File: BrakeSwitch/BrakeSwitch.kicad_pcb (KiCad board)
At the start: 2 copper layers, 16 parts, among them Q1 NMOS, U1 XL1509-5.0, U2 LMV321, U3 LMV321

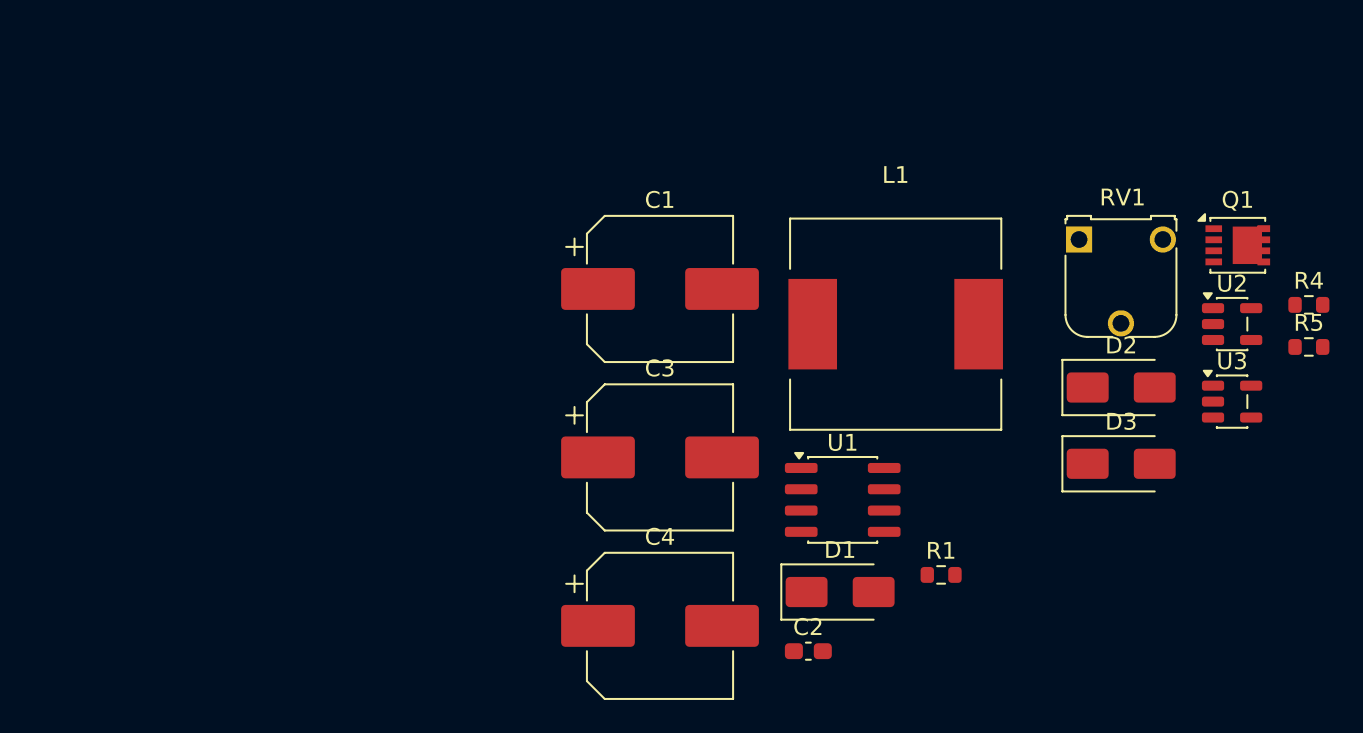
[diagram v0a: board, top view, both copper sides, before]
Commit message: Basic layout done
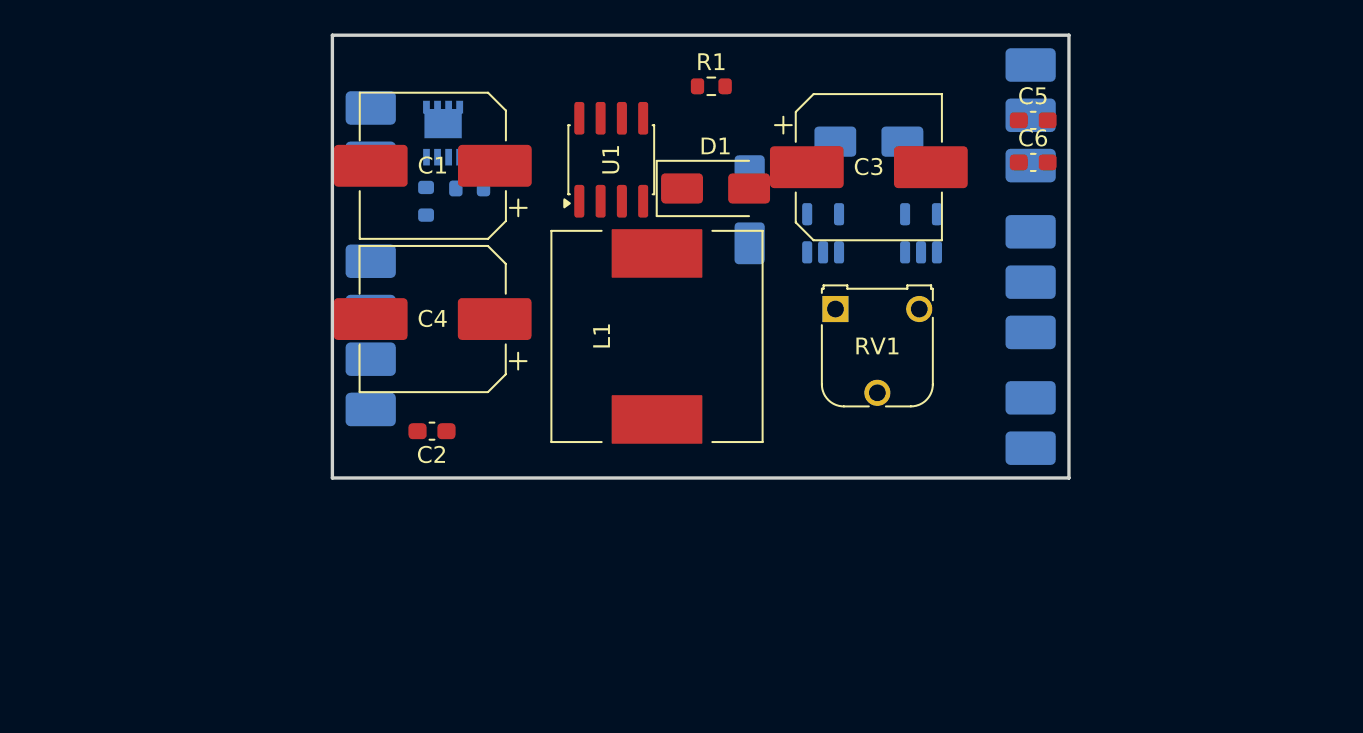
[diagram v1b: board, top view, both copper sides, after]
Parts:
- added C5: 1u, Capacitor_SMD:C_0603_1608Metric_Pad1.08x0.95mm_HandSolder, F.Cu at (114.2, 38.9)
- added C6: 1u, Capacitor_SMD:C_0603_1608Metric_Pad1.08x0.95mm_HandSolder, F.Cu at (114.2, 41.4)
- added J1: 12V_in, AA-Custom:SolderPad_01x02, B.Cu at (74.7, 48.8)
- added J2: LightPlug, AA-Custom:SolderPad_01x02, B.Cu at (74.7, 39.6)
- added J3: 5V_out, AA-Custom:SolderPad_01x02, B.Cu at (114.0, 56.9)
- added J4: Front_Pads, AA-Custom:SolderPad_01x03, B.Cu at (114.0, 48.5)
- added J5: Back_Pads, AA-Custom:SolderPad_01x03, B.Cu at (114.0, 38.6)
- added J6: 12V_in, AA-Custom:SolderPad_01x02, B.Cu at (74.7, 54.6)
- D2, D3, Q1, R4, R5, U2, U3: moved to B.Cu
- moved R5 53.4 mm to (78.0, 43.7), turned to -90 degrees
- moved R4 50.5 mm to (80.6, 42.9), turned to 180 degrees
- moved Q1 47.9 mm to (79.0, 39.6), turned to 90 degrees
- moved R1 32.2 mm to (95.0, 36.8)
- moved C2 26.0 mm to (78.3, 57.4), turned to 180 degrees
- moved D1 25.2 mm to (95.2, 42.9)
- moved U2 25.0 mm to (101.7, 45.6), turned to 90 degrees
- moved D2 24.6 mm to (97.3, 44.2), turned to -90 degrees
- moved U1 24.5 mm to (89.0, 41.2), turned to 90 degrees
- moved D3 24.4 mm to (104.4, 40.1)
- moved C4 22.8 mm to (78.4, 50.7), turned to 180 degrees
- moved C3 21.3 mm to (104.4, 41.7)
- moved U3 21.1 mm to (107.5, 45.6), turned to 90 degrees
- moved C1 15.4 mm to (78.4, 41.6), turned to 180 degrees
- moved RV1 15.1 mm to (102.4, 50.1)
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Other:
- board outline added: 43.9 x 26.4 mm

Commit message: Some feedback and layout
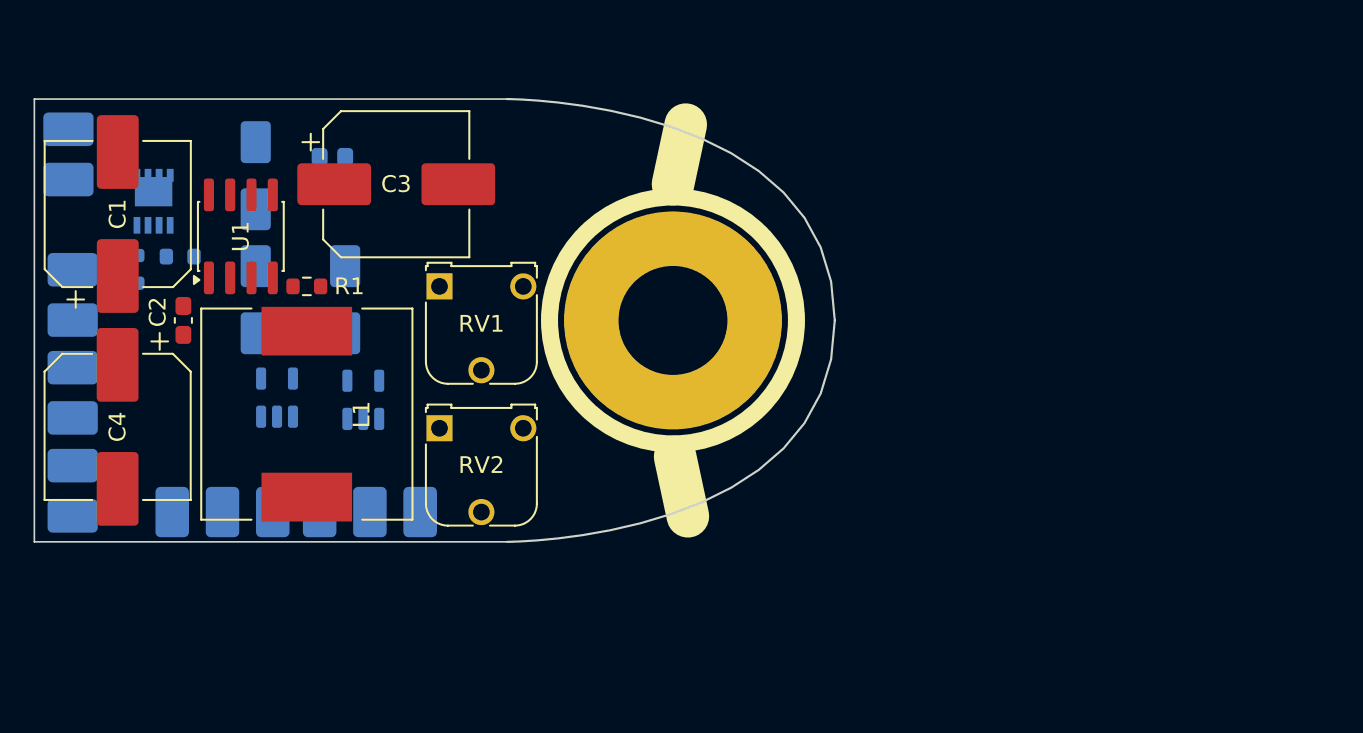
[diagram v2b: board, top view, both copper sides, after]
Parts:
- added H1: MountingHole, MountingHole:MountingHole_6.5mm_Pad, F.Cu at (92.7, 50.8)
- added RV2: Thresh, Potentiometer_THT:Potentiometer_Runtron_RM-065_Vertical, F.Cu at (78.8, 57.2)
- C5, C6, D1: moved to B.Cu
- J4: value Front_Pads -> Front_Loop
- J5: value Back_Pads -> Rear_Loop
- J6: value 12V_in -> 12V_Out
- moved J3 57.7 mm to (56.9, 49.3)
- moved J5 53.7 mm to (65.8, 62.2), turned to 180 degrees
- moved C5 42.7 mm to (71.6, 41.9), turned to -90 degrees
- moved J4 41.7 mm to (74.6, 62.2), turned to 180 degrees
- moved C6 41.1 mm to (73.2, 41.9), turned to -90 degrees
- moved U3 39.7 mm to (69.1, 55.4)
- moved D3 37.8 mm to (67.8, 49.6), turned to -90 degrees
- moved U2 29.2 mm to (74.2, 55.5)
- moved C3 28.2 mm to (76.2, 42.7)
- moved D1 27.4 mm to (67.8, 42.2), turned to 90 degrees
- moved R1 26.9 mm to (70.9, 48.8)
- moved D2 24.7 mm to (73.2, 49.6)
- moved RV1 23.7 mm to (78.8, 48.8)
- moved U1 22.6 mm to (66.9, 45.8)
- moved L1 21.4 mm to (70.9, 56.4), turned to -90 degrees
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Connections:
- C1 pad 1: /DCDC/Vin -> 12V
- C2 pad 1: /DCDC/Vin -> 12V
- C4 pad 1: /DCDC/Vin -> 12V
- U1 pad 1: /DCDC/Vin -> 12V
- U3 pad 3: Net-(U2--) -> Net-(U3--)
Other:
- board size 43.9 x 26.4 mm -> 47.8 x 26.4 mm
- board text added: "Diddy's Minion RIT Baja 3/19/2026"
